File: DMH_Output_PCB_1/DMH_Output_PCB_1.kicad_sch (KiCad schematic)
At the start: 0 parts

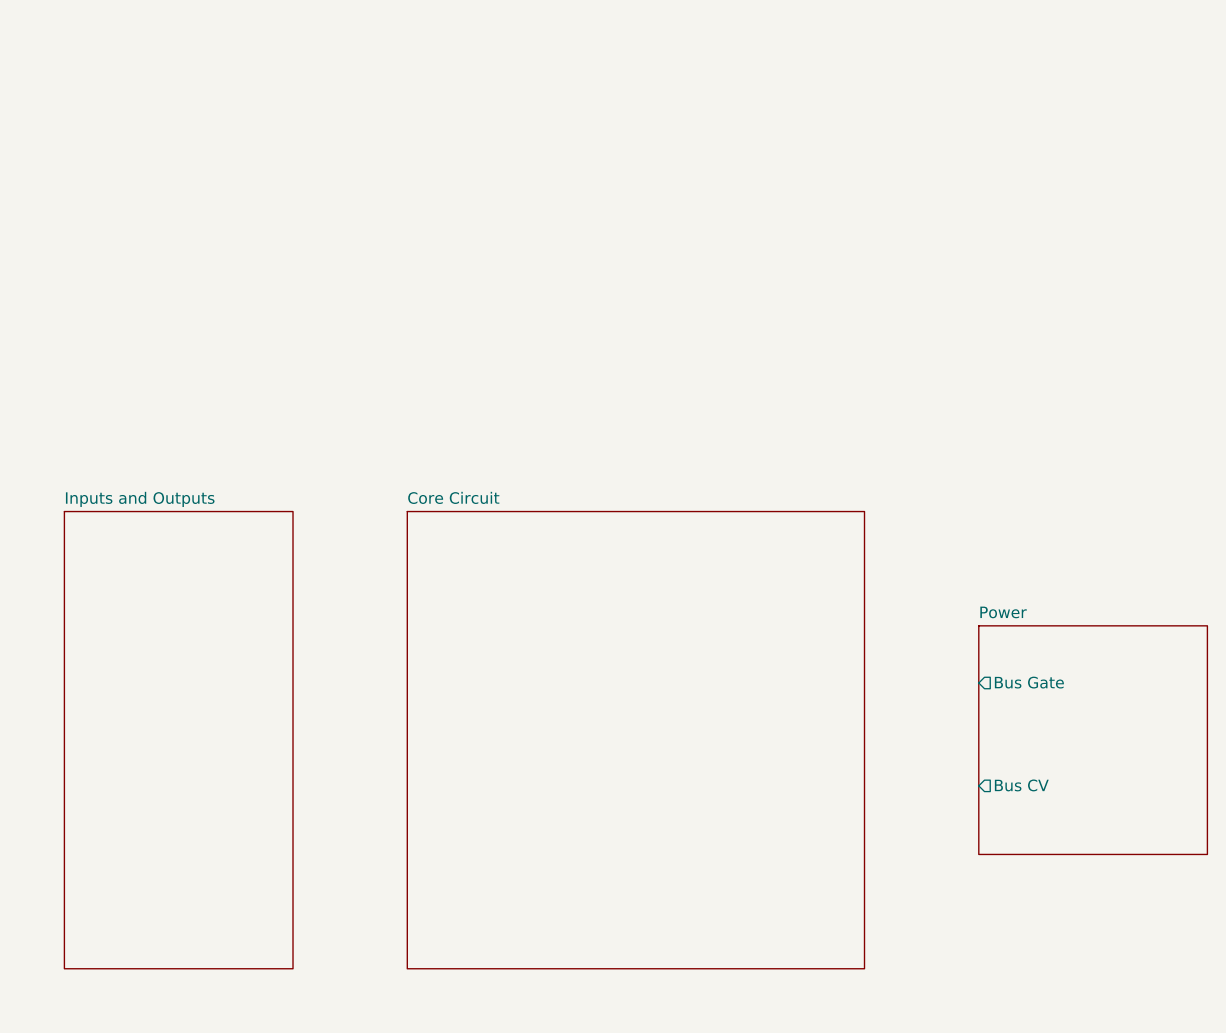
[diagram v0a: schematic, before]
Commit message: Schematic in progress
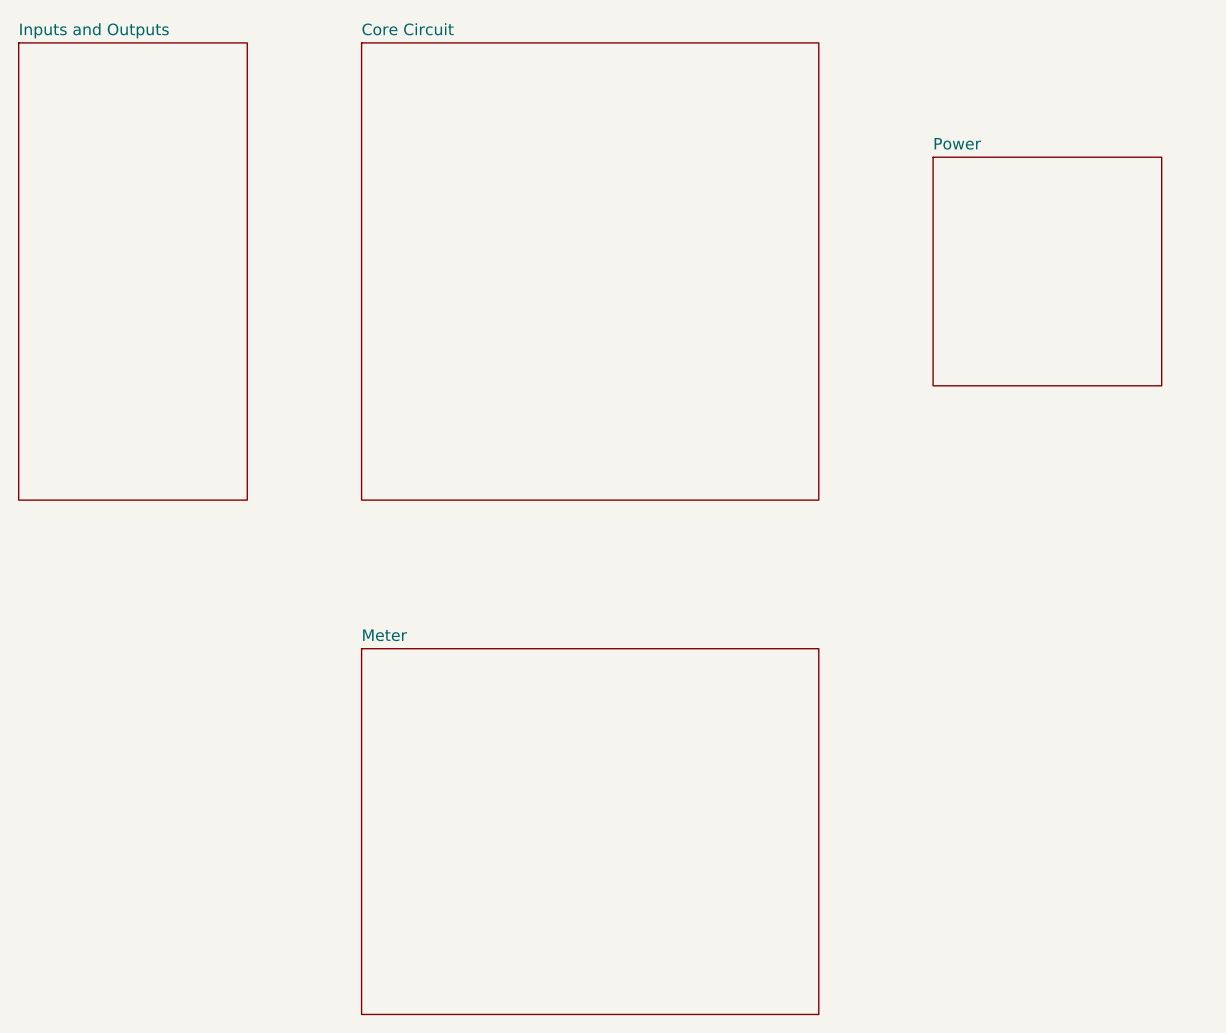
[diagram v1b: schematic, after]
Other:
- added sheet Meter (Meter.kicad_sch)
- sheet Power ports: added none; removed Bus CV, Bus Gate
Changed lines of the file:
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@@
 	)
 	(sheet
-		(at 127 88.9)
+		(at 121.92 36.83)
 		(size 25.4 25.4)
 		(exclude_from_sim no)
@@
 		)
 		(property "Sheetname" "Power"
-			(at 127 88.1884 0)
+			(at 121.92 36.1184 0)
 			(effects
 				(font
@@
 		)
 		(property "Sheetfile" "Power.kicad_sch"
-			(at 127 114.8846 0)
+			(at 121.92 62.8146 0)
 			(effects
 				(font
@@
 			)
 		)
-		(pin "Bus Gate" output
-			(at 127 95.25 180)
-			(effects
-				(font
-					(size 1.27 1.27)
-				)
-				(justify left)
-			)
-		)
-		(pin "Bus CV" output
-			(at 127 106.68 180)
-			(effects
-				(font
-					(size 1.27 1.27)
-				)
-				(justify left)
-			)
-		)
 		(instances
-			(project "DMH-Kosmo-5cm-PCB"
+			(project "DMH_Output_PCB_1"
 				(path "/58f4306d-5387-4983-bb08-41a2313fd315"
 					(page "4")
@@
 	)
 	(sheet
-		(at 63.5 76.2)
+		(at 58.42 24.13)
 		(size 50.8 50.8)
 		(exclude_from_sim no)
@@
 		)
 		(property "Sheetname" "Core Circuit"
-			(at 63.5 75.4884 0)
+			(at 58.42 23.4184 0)
 			(effects
 				(font
@@
 		)
 		(property "Sheetfile" "Core_Circuit.kicad_sch"
-			(at 63.5 127.5846 0)
+			(at 58.42 75.5146 0)
 			(effects
 				(font
@@
 		)
 		(instances
-			(project "DMH-Kosmo-5cm-PCB"
+			(project "DMH_Output_PCB_1"
 				(path "/58f4306d-5387-4983-bb08-41a2313fd315"
 					(page "3")
@@
 	)
 	(sheet
-		(at 25.4 76.2)
+		(at 58.42 91.44)
+		(size 50.8 40.64)
+		(exclude_from_sim no)
+		(in_bom yes)
+		(on_board yes)
+		(dnp no)
+		(fields_autoplaced yes)
+		(stroke
+			(width 0.1524)
+			(type solid)
+		)
+		(fill
+			(color 0 0 0 0.0000)
+		)
+		(property "Sheetname" "Meter"
+			(at 58.42 90.7284 0)
+			(effects
+				(font
+					(size 1.27 1.27)
+				)
+				(justify left bottom)
+			)
+		)
+		(property "Sheetfile" "Meter.kicad_sch"
+			(at 58.42 132.6646 0)
+			(effects
+				(font
+					(size 1.27 1.27)
+				)
+				(justify left top)
+				(hide yes)
+			)
+		)
+		(instances
+			(project "DMH_Output_PCB_1"
+				(path "/58f4306d-5387-4983-bb08-41a2313fd315"
+					(page "5")
+				)
+			)
+		)
+	)
+	(sheet
+		(at 20.32 24.13)
 		(size 25.4 50.8)
 		(exclude_from_sim no)
@@
 		)
 		(property "Sheetname" "Inputs and Outputs"
-			(at 25.4 75.4884 0)
+			(at 20.32 23.4184 0)
 			(effects
 				(font
@@
 		)
 		(property "Sheetfile" "Inputs_and_Outputs.kicad_sch"
-			(at 25.4 127.5846 0)
+			(at 20.32 75.5146 0)
 			(effects
 				(font
@@
 		)
 		(instances
-			(project "DMH-Kosmo-5cm-PCB"
+			(project "DMH_Output_PCB_1"
 				(path "/58f4306d-5387-4983-bb08-41a2313fd315"
 					(page "2")
